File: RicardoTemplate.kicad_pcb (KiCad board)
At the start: 4 copper layers, 42.8 x 63.6 mm, 143 parts, among them IC2 SX1280, J1 RBUS, J2 USB_C_Receptacle_USB2.0, U1 ESP32-S3, U11 SC4215ASTRT, U12 SKY66112-11, U13 DEA202450BT-1213C1, U2 SN65HVD230, U3 LM66200DRLR, U4 MAX77827AEFD+T, U5 SC4215ASTRT, Y1 R940000171, Y3 Crystal_GND24

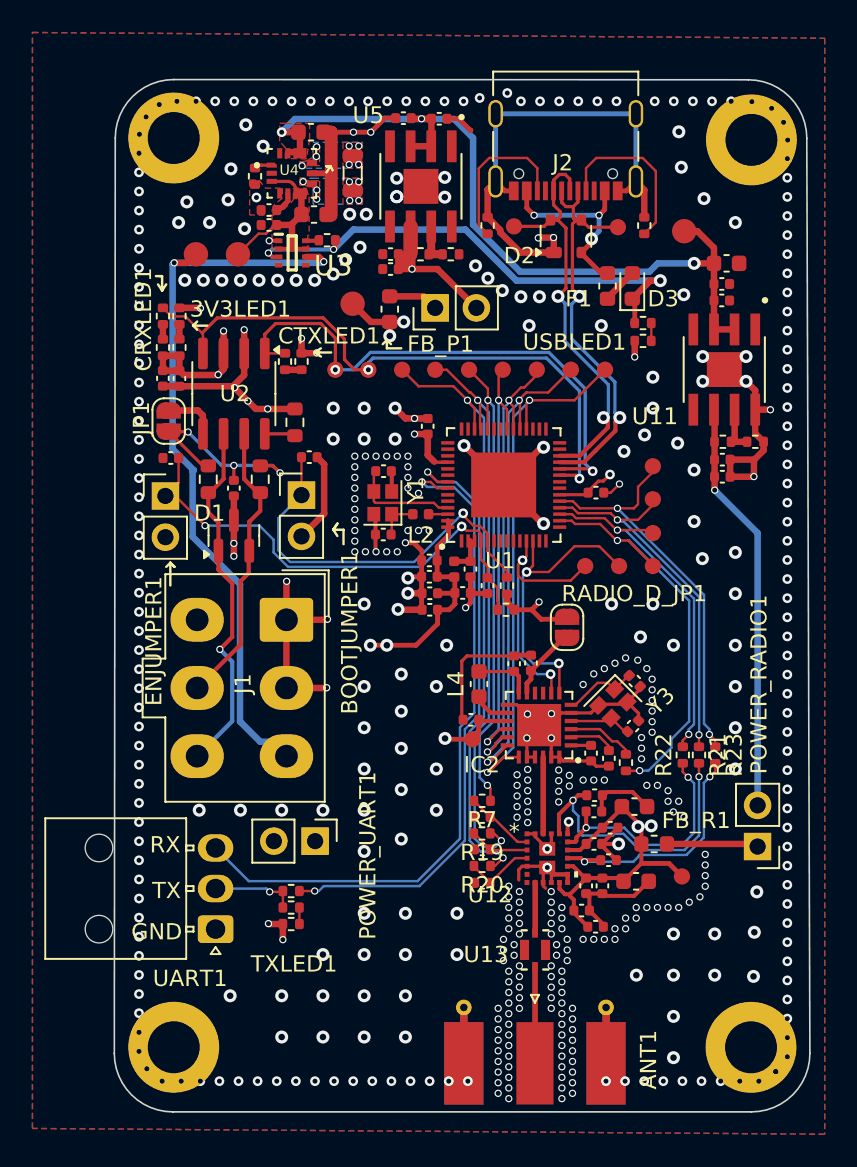
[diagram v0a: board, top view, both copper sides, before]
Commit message: Minor improvements
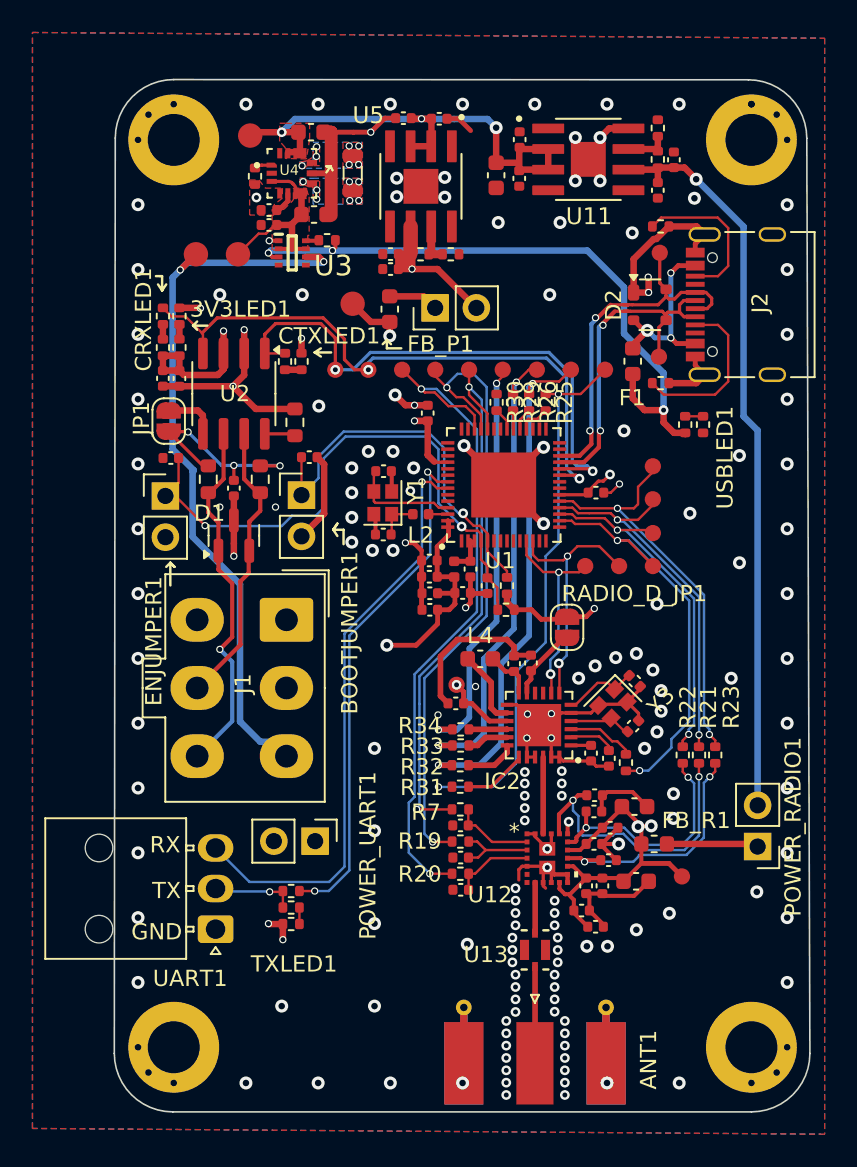
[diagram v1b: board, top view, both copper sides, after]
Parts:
- removed D3: D, Diode_SMD:D_0603_1608Metric
- added R25: 20-100, Resistor_SMD:R_0402_1005Metric, F.Cu at (145.0, 90.9)
- added R26: 20-100, Resistor_SMD:R_0402_1005Metric, F.Cu at (144.0, 90.9)
- added R29: 20-100, Resistor_SMD:R_0402_1005Metric, F.Cu at (143.0, 90.9)
- added R30: 20-100, Resistor_SMD:R_0402_1005Metric, F.Cu at (142.0, 90.9)
- added R31: 20-100, Resistor_SMD:R_0402_1005Metric, F.Cu at (139.8, 114.5)
- added R32: 20-100, Resistor_SMD:R_0402_1005Metric, F.Cu at (139.8, 113.2)
- added R33: 20-100, Resistor_SMD:R_0402_1005Metric, F.Cu at (139.8, 112.0)
- added R34: 20-100, Resistor_SMD:R_0402_1005Metric, F.Cu at (139.8, 111.0)
- moved BBOUT_TP1 27.4 mm to (126.8, 74.4)
- moved R28 20.2 mm to (151.9, 74.0), turned to 90 degrees
- moved C64 19.7 mm to (152.9, 75.9), turned to -90 degrees
- moved R27 17.8 mm to (151.9, 75.9), turned to 90 degrees
- moved C62 17.1 mm to (151.9, 77.8), turned to 90 degrees
- moved C19 15.9 mm to (143.4, 74.7), turned to 90 degrees
- moved U11 15.4 mm to (147.7, 75.9), turned to 0 degrees
- moved C12 15.2 mm to (142.0, 76.9), turned to -90 degrees
- moved J2 14.2 mm to (156.8, 84.8), turned to 90 degrees
- moved C18 14.1 mm to (143.4, 77.1), turned to -90 degrees
- moved R12 10.7 mm to (152.1, 80.0), turned to 180 degrees
- moved R11 9.76 mm to (152.1, 89.7), turned to 0 degrees
- moved D+_TP1 9.13 mm to (152.1, 81.7), turned to -90 degrees
- moved D-_TP1 8.37 mm to (152.0, 88.1), turned to -90 degrees
- moved R13 6.77 mm to (153.6, 92.2), turned to 90 degrees
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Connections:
- F1 pad 2: Net-(D3-A) -> VBUS
- IC2 pad 16: MISO -> Net-(IC2-MISO_TX)
- IC2 pad 17: MOSI -> Net-(IC2-MOSI_RX)
- IC2 pad 18: SCK -> Net-(IC2-SCK_RTSN)
- IC2 pad 19: CS -> Net-(IC2-NSS_CTS)
- U1 pad 32: CS -> Net-(U1-SPICS0/GPIO29)
- U1 pad 33: SCK -> Net-(U1-SPICLK/GPIO30)
- U1 pad 34: MOSI -> Net-(U1-SPIQ/GPIO31)
- U1 pad 35: MISO -> Net-(U1-SPID/GPIO32)
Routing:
- net Net-(POWER_RADIO1-Pin_2): track 25.5 -> 45.6 mm
- net +VDC: track 50.0 -> 32.9 mm
- net GND: track 398.5 -> 382.4 mm, vias 478 -> 178
- net VBUS: track 31.3 -> 39.2 mm
- net /RXD: track 43.4 -> 36.6 mm
- net Net-(U1-U0TXD/PROG/GPIO43): track 38.0 -> 31.7 mm
- net /CHIP_PU: track 30.7 -> 36.5 mm
- net CRX: track 29.6 -> 34.3 mm
- net Net-(IC2-NSS_CTS): track 0.00 -> 3.92 mm
- net ANT_SEL: track 38.1 -> 42.0 mm
- net DIO1: track 16.6 -> 12.8 mm
- net /Data-: track 25.3 -> 21.5 mm
- net CSD: track 35.8 -> 39.4 mm
- net Net-(IC2-SCK_RTSN): track 0.00 -> 3.13 mm
- net /Data+: track 25.9 -> 22.9 mm
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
